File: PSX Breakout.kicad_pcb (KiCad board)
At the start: 2 copper layers, 100 x 51.8 mm, 30 parts, among them J1 Conn_01x12_Male, J2 Mini-DIN-4, J3 VAL**, J4 DB15_Female_HighDensity, J5 3x2_RCA, SW1 SW_SPDT, SW2 SW_SP3T, SW3 SW_SP3T, U1 LM1881

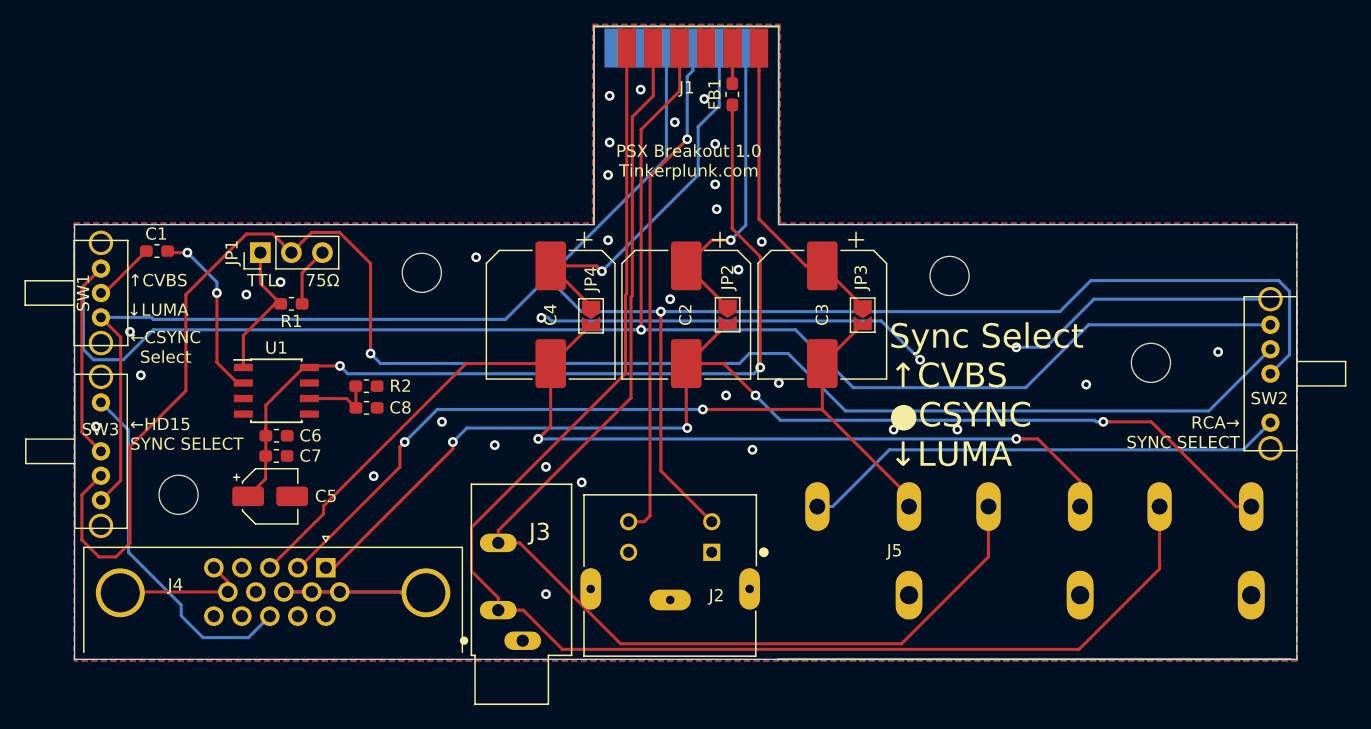
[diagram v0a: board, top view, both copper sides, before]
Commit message: Fixing Merging Error
Updated Case, moved connector, generated gerbers
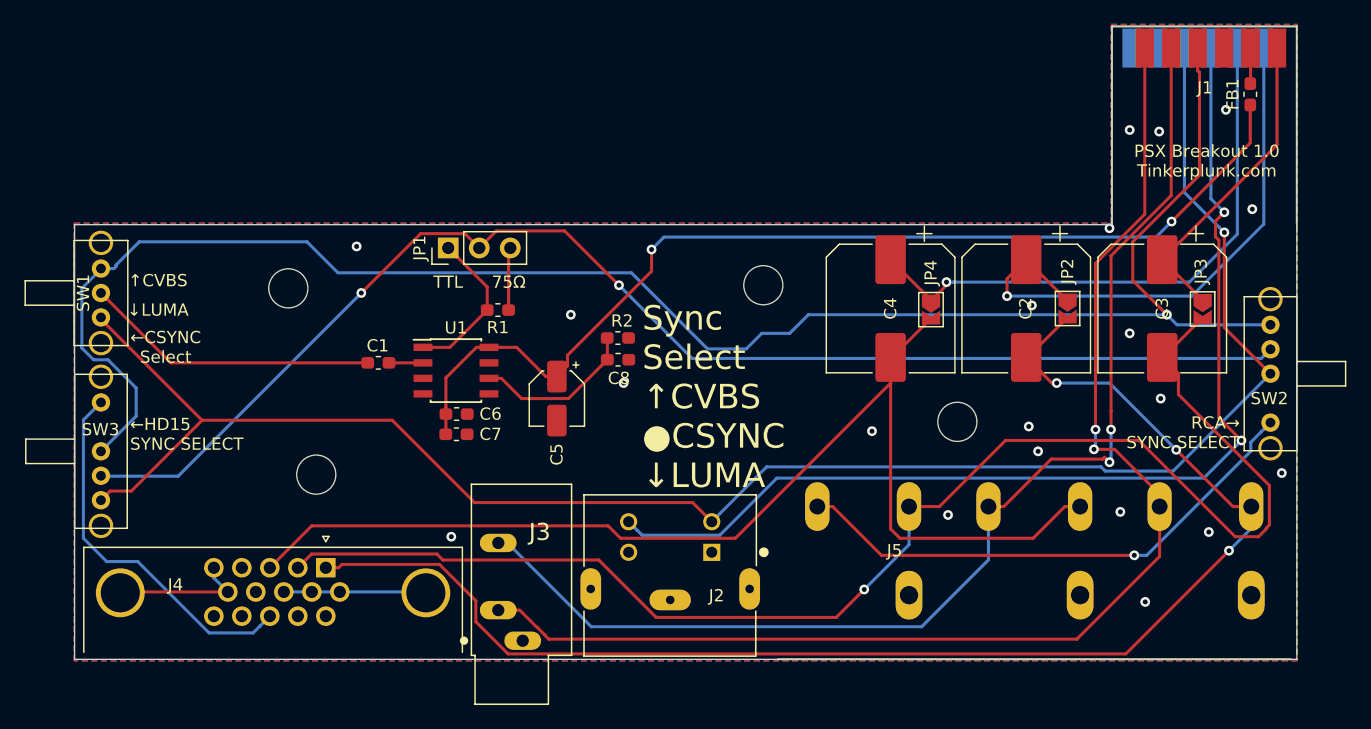
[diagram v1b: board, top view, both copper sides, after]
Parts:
- removed BTM: Case_BTM, PSX_BREAKOUT:Case_BTM
- removed the REF** at (98.5, 98.3)
- removed the REF** at (118.4, 80.1)
- removed the REF** at (161.5, 80.4)
- removed the REF** at (178.0, 87.5)
- removed TOP: Case_TOP, PSX_BREAKOUT:Case_TOP
- added REF**: MountingHole_3.2mm_M3, MountingHole:MountingHole_3.2mm_M3, F.Cu at (109.7, 96.6)
- added REF**: MountingHole_3.2mm_M3, MountingHole:MountingHole_3.2mm_M3, F.Cu at (107.4, 81.4)
- added REF**: MountingHole_3.2mm_M3, MountingHole:MountingHole_3.2mm_M3, F.Cu at (162.2, 92.3)
- added REF**: MountingHole_3.2mm_M3, MountingHole:MountingHole_3.2mm_M3, F.Cu at (146.3, 81.2)
- moved FB1 42.4 mm to (186.1, 65.5)
- moved J1 42.4 mm to (182.4, 60.0)
- moved C3 27.8 mm to (178.9, 83.1)
- moved JP3 27.8 mm to (182.2, 83.1)
- moved JP4 27.8 mm to (160.0, 83.1)
- moved C2 27.8 mm to (167.8, 83.1)
- moved C4 27.8 mm to (156.7, 83.1)
- moved JP2 27.8 mm to (171.2, 83.1)
- moved C5 24.8 mm to (129.4, 90.4), turned to 270 degrees
- moved C8 20.9 mm to (134.4, 87.2)
- moved R2 20.9 mm to (134.4, 85.5)
- moved C1 20.3 mm to (114.8, 87.5)
- moved R1 16.9 mm to (124.6, 83.2)
- moved JP1 15.4 mm to (120.5, 78.1)
- moved C6 14.8 mm to (121.2, 91.7)
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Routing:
- net GND: track 87.3 -> 22.9 mm, vias 35 -> 20
- net GREEN_OUT: track 68.5 -> 115.6 mm, vias 2 -> 1
- net CHROMA: track 41.7 -> 87.5 mm, vias 1 -> 2
- net CSYNC: track 138.3 -> 109.6 mm, vias 1 -> 2
- net RED_OUT: track 95.7 -> 117.2 mm, vias 4 -> 3
- net RED: track 25.5 -> 46.2 mm
- net Net-(C1-Pad2): track 5.13 -> 24.2 mm
- net LUMA: track 166.9 -> 148.5 mm
- net BLUE: track 31.3 -> 47.4 mm
- net Net-(C5-Pad1): track 72.9 -> 85.0 mm
- net Net-(C1-Pad1): track 14.5 -> 2.77 mm, vias 2 -> 0
- net RIGHT: track 115.4 -> 104.4 mm, vias 0 -> 2
- net Net-(C8-Pad1): track 5.90 -> 13.5 mm
- net BLUE_OUT: track 89.3 -> 95.5 mm, vias 2 -> 0
- net CVBS: track 150.4 -> 146.4 mm
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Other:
- outline, holes or cut-outs redrawn
